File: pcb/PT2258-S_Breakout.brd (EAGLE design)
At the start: 54 x 51.5 mm, 41 parts, among them U1 PT2258-S, X1 INPUT, X2 I2C, X3 POWER, X4 OUTPUT

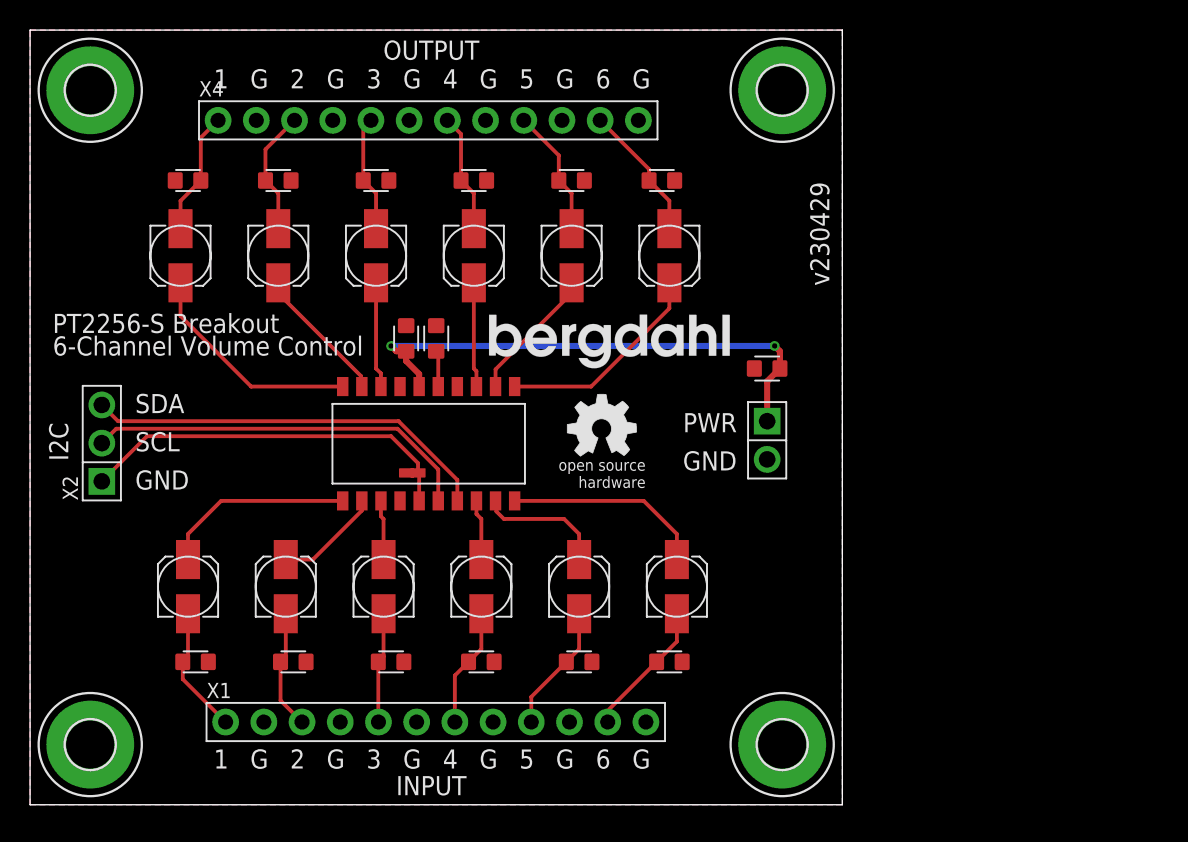
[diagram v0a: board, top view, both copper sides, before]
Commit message: Final version
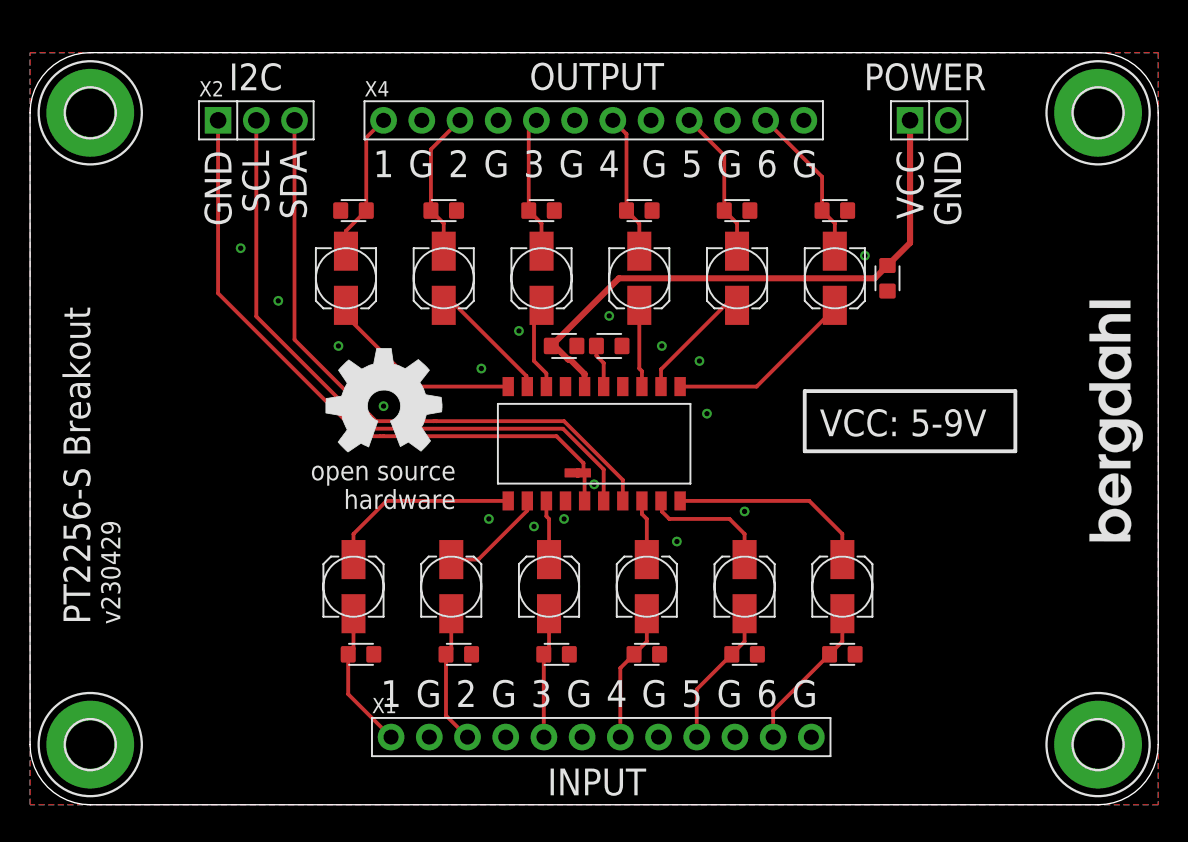
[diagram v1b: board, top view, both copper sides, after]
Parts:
- removed U$4: (no value), M2M-Frames:OSHW-5MM-TPLACE
- added U$5: (no value), M2M-Frames:OSHW-8MM-TPLACE
- moved U$3 45.0 mm to (74.0, 17.5), turned to 90 degrees
- moved X2 25.2 mm to (12.5, 45.5), turned to 0 degrees
- moved X3 22.1 mm to (58.5, 45.5), turned to 0 degrees
- moved H3 21.1 mm to (71.0, 46.0)
- moved H4 21.0 mm to (71.0, 4.00)
- moved R12 11.7 mm to (53.5, 39.5)
- moved C8 11.5 mm to (38.5, 30.5), turned to 0 degrees
- moved R6 11.5 mm to (54.0, 10.0)
- moved R10 11.2 mm to (40.5, 39.5)
- moved R11 11.2 mm to (47.0, 39.5)
- moved R7 11.2 mm to (21.5, 39.5)
- moved R8 11.2 mm to (27.5, 39.5)
- moved R9 11.2 mm to (34.0, 39.5)
- moved C10 11.1 mm to (21.0, 35.0)
- moved C11 11.1 mm to (27.5, 35.0)
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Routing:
- net GND: track 25.5 -> 43.0 mm
- net SCL: track 26.0 -> 42.4 mm
- net SDA: track 27.1 -> 41.7 mm
- net VCC: track 34.9 -> 38.7 mm, vias 2 -> 0
- net N$11: track 6.97 -> 5.47 mm
- net N$2: track 8.35 -> 9.85 mm
- net N$1: track 8.24 -> 9.74 mm
- net N$9: track 14.1 -> 12.6 mm
- net N$5: track 8.52 -> 10.0 mm
- net N$14: track 14.9 -> 13.4 mm
- net N$6: track 9.11 -> 10.6 mm
- net N$4: track 7.93 -> 9.43 mm
- net N$3: track 7.76 -> 9.26 mm
- net N$12: track 7.03 -> 5.95 mm
- net N$13: track 9.20 -> 8.17 mm
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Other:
- board size 54 x 51.5 mm -> 75 x 50 mm
- board text added: "POWER"
- board text added: "VCC"
- board text added: "VCC: 5-9V"
- board text removed: "6-Channel Volume Control"
- board text removed: "PWR"
